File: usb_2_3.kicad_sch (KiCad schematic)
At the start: 20 parts, among them J4 USB3_A_Stacked, J5 USB_A_Stacked, U3 D3V3XA4B10LP, U4 D3V3XA4B10LP

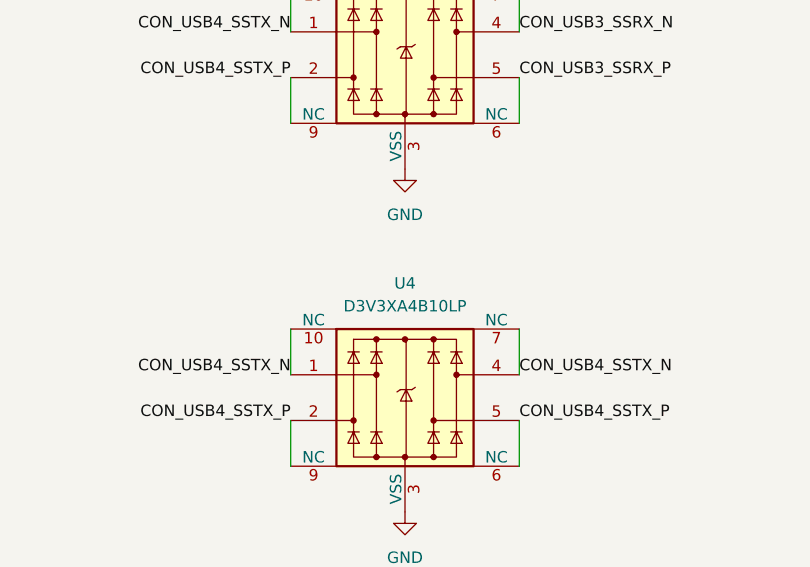
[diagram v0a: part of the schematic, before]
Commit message: Designators in GPIO restored
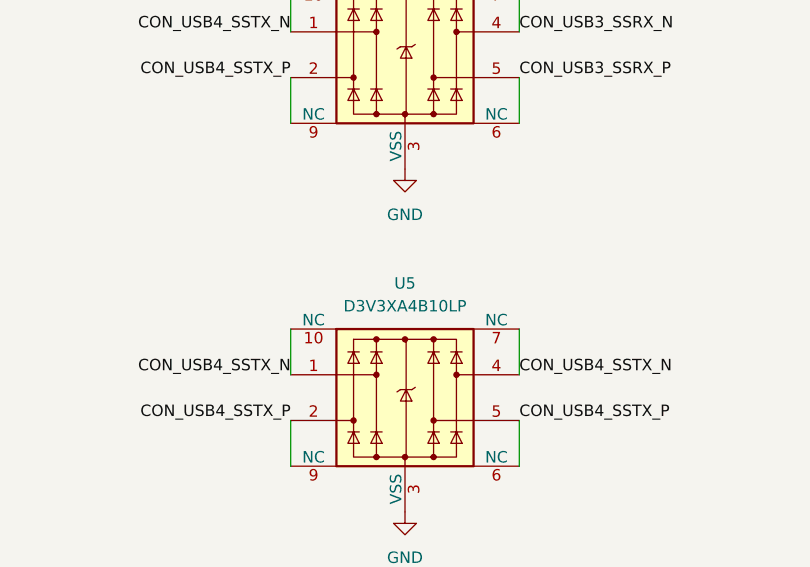
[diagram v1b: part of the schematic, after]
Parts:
- renumbered U4 to U5
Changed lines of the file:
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@@
 		(dnp no)
 		(fields_autoplaced yes)
-		(property "Reference" "U4"
+		(property "Reference" "U5"
 			(at 67.31 156.21 0)
 			(show_name no)
@@
 			(project "Carrier_Board"
 				(path "/e768274e-12f3-4f83-96f6-abb7638e0bc1/f6805346-90aa-47cf-a186-fe5806ffb5a5"
-					(reference "U4")
+					(reference "U5")
 					(unit 1)
 				)
